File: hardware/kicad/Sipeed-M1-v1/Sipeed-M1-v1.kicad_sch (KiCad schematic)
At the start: 167 parts, among them IC1 TROPIC01_chip, J1 USB_C_, J2 JST Connector, J3 Conn_02x20_Odd_Even, J4 Conn_01x09_Pin, J5 Conn_02x03_Odd_Even, Q2 FS8205A, SW1 SW_Push, SW10 SW_Push, SW11 SW_Push, SW12 SW_Push, SW13 SW_Push, SW14 SW_Push, SW15 SW_Push, SW16 SW_Push, SW2 SW_Push, SW3 SW_Push, SW4 SW_Push, SW5 SW_Push, SW6 SW_Push, SW7 SW_Push, SW8 SW_Push, SW9 SW_Push, U1 Sipeed-M1, U2 ESP32-S3-WROOM-1U-N8R8, U3 PAM2401YPADJ, U4 TPS63070RNMR, U5 MCP23017_SO, U6 BQ29700DSER, U7 USBLC6-2SC6, U8 MCP73871

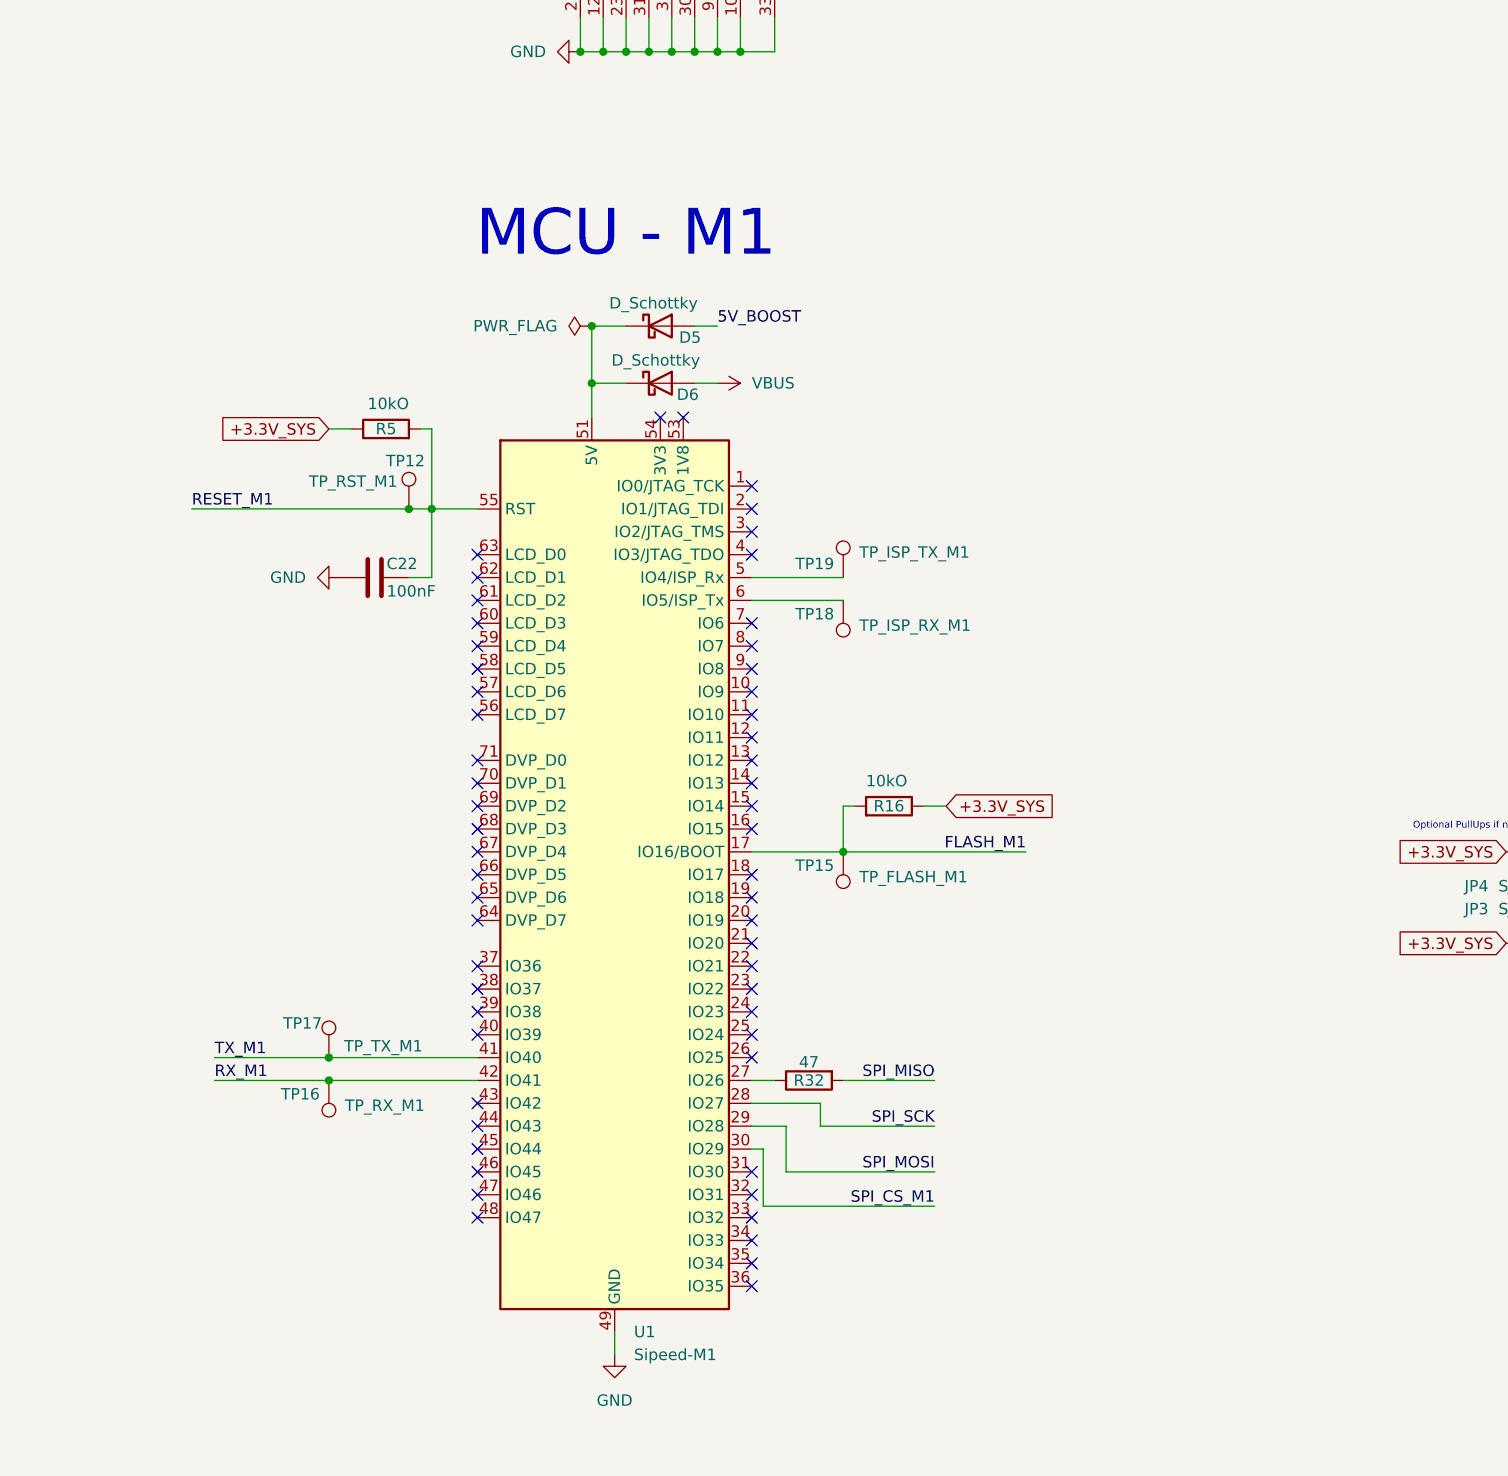
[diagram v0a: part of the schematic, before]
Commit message: adding M1 changes
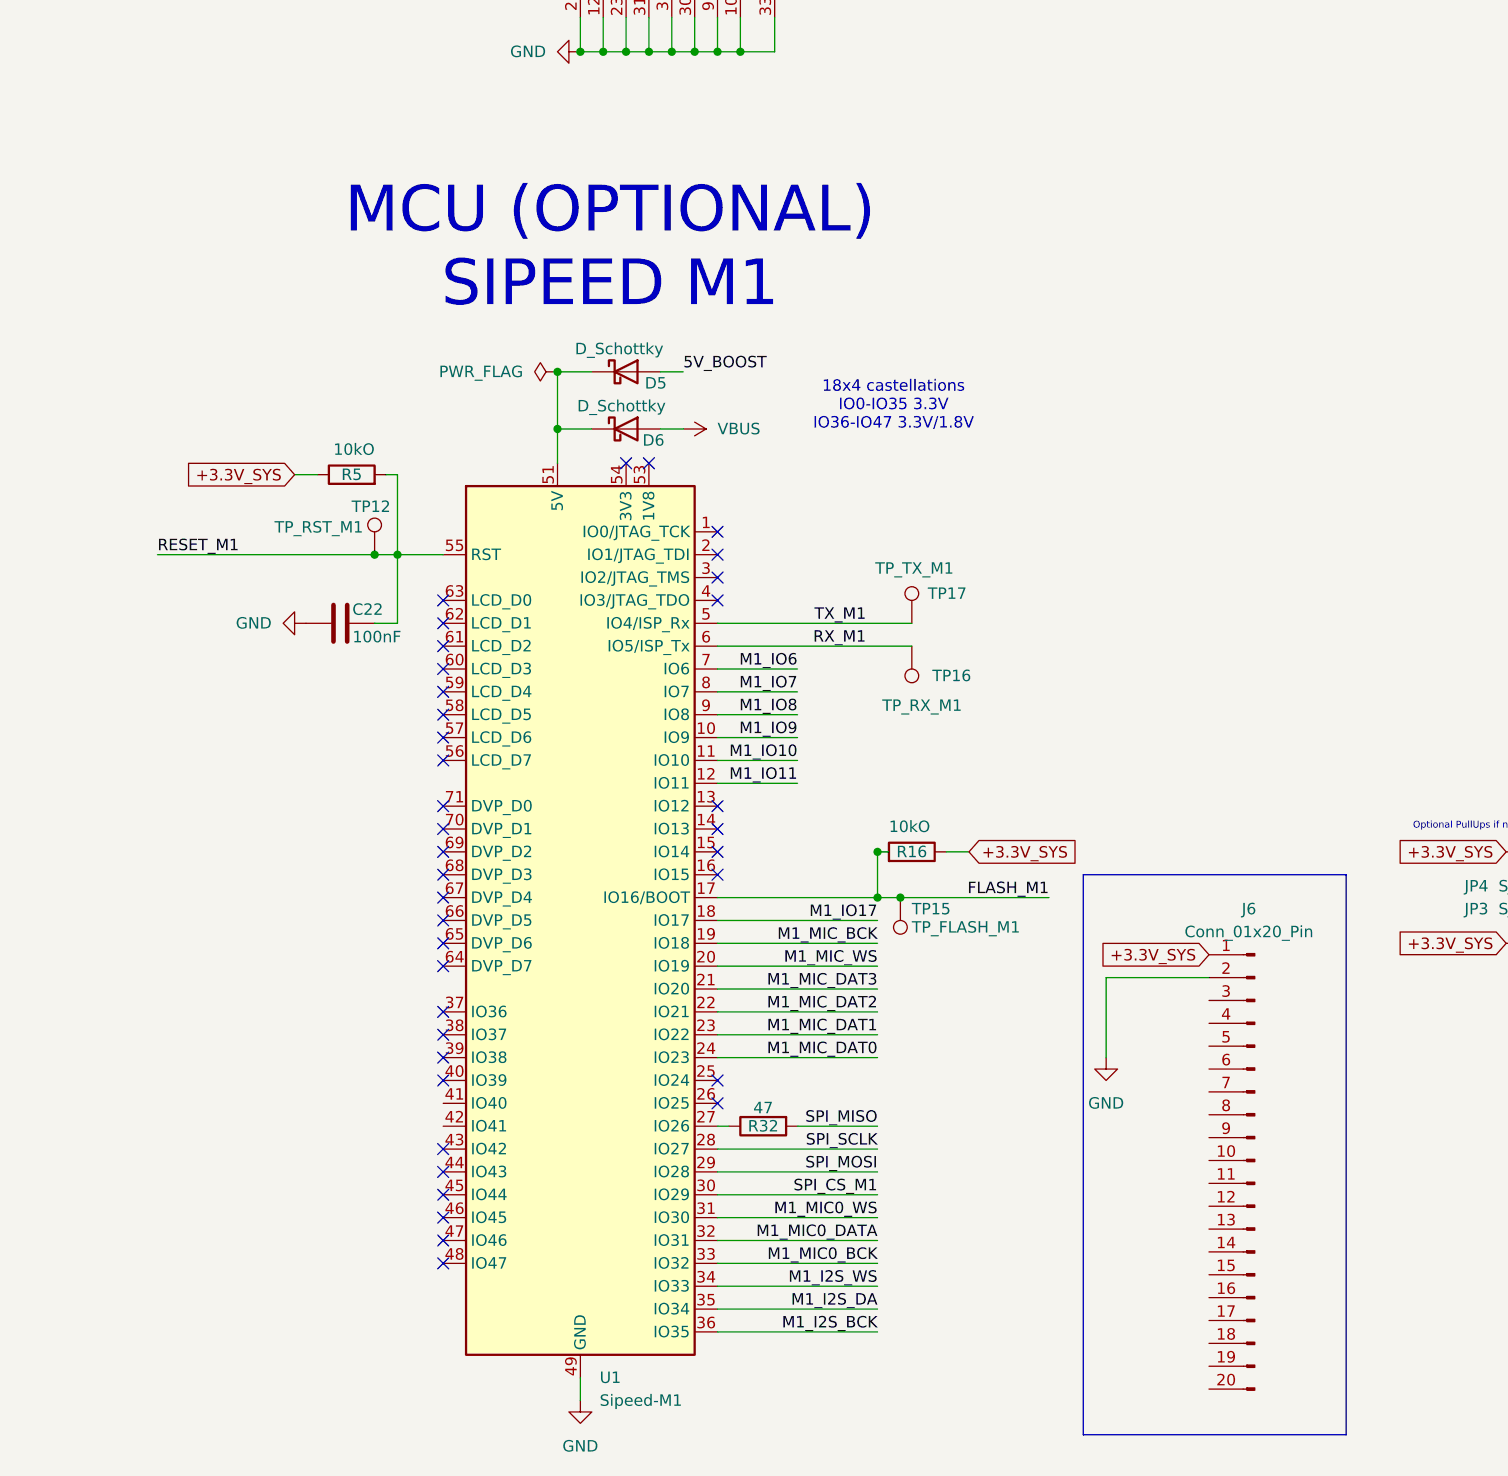
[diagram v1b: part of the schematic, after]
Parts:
- removed TP18: TP_ISP_RX_M1, TestPoint:TestPoint_Pad_D2.0mm, symbol Connector:TestPoint
- removed TP19: TP_ISP_TX_M1, TestPoint:TestPoint_Pad_D2.0mm, symbol Connector:TestPoint
- added J6: Conn_01x20_Pin, symbol Connector:Conn_01x20_Pin
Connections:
- net +3.3V_SYS: now also J6.1 (Pin_1)
- net GND: now also J6.2 (Pin_2)
- net RX_M1: now also U1.6 (IO5/ISP_Tx); no longer U1.42 (IO41)
- net SPI_SCK: no longer U1.28 (IO27)
- net TX_M1: now also U1.5 (IO4/ISP_Rx); no longer U1.41 (IO40)
- net M1_IO9: now reaches U1.10 (IO9)
- net M1_IO10: now reaches U1.11 (IO10)
- net M1_IO11: now reaches U1.12 (IO11)
- net M1_IO17: now reaches U1.18 (IO17)
- net M1_MIC_BCK: now reaches U1.19 (IO18)
- net M1_MIC_WS: now reaches U1.20 (IO19)
- net M1_MIC_DAT3: now reaches U1.21 (IO20)
- net M1_MIC_DAT2: now reaches U1.22 (IO21)
- net M1_MIC_DAT1: now reaches U1.23 (IO22)
- net M1_MIC_DAT0: now reaches U1.24 (IO23)
- net M1_MIC0_WS: now reaches U1.31 (IO30)
- net M1_MIC0_DATA: now reaches U1.32 (IO31)
- net M1_MIC0_BCK: now reaches U1.33 (IO32)
- net M1_I2S_WS: now reaches U1.34 (IO33)
- net M1_I2S_DA: now reaches U1.35 (IO34)
- net M1_I2S_BCK: now reaches U1.36 (IO35)
- net M1_IO6: now reaches U1.7 (IO6)
- net M1_IO7: now reaches U1.8 (IO7)
- net M1_IO8: now reaches U1.9 (IO8)
- new net SPI_SCLK: U1.28 (IO27)
- no-connect marks 62 -> 43
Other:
- note added: "18x4 castellations IO0-IO35 3.3V IO36-IO47 3.3V/1.8V"
- note added: "MCU (OPTIONAL) SIPEED M1"
- note removed: "MCU - M1"
- moved on the sheet: C22, D5, D6, R16, R32, R5, TP12, TP15, TP16, TP17, U1

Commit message: power symbol fix
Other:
- note added: "Secure Element TROPIC01"
- note removed: "Secure Element - TROPIC01"
- moved on the sheet: C25, C26, C27, C28, IC1, R34, R48
